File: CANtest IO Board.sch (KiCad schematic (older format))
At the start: 40 parts, among them J1 Inputs, J2 Conn_02x16_Counter_Clockwise, J3 Outputs, SW1 SW_SPDT_MSM, SW2 SW_SPST, SW3 SW_SPST, SW4 SW_Push, SW5 SW_Push

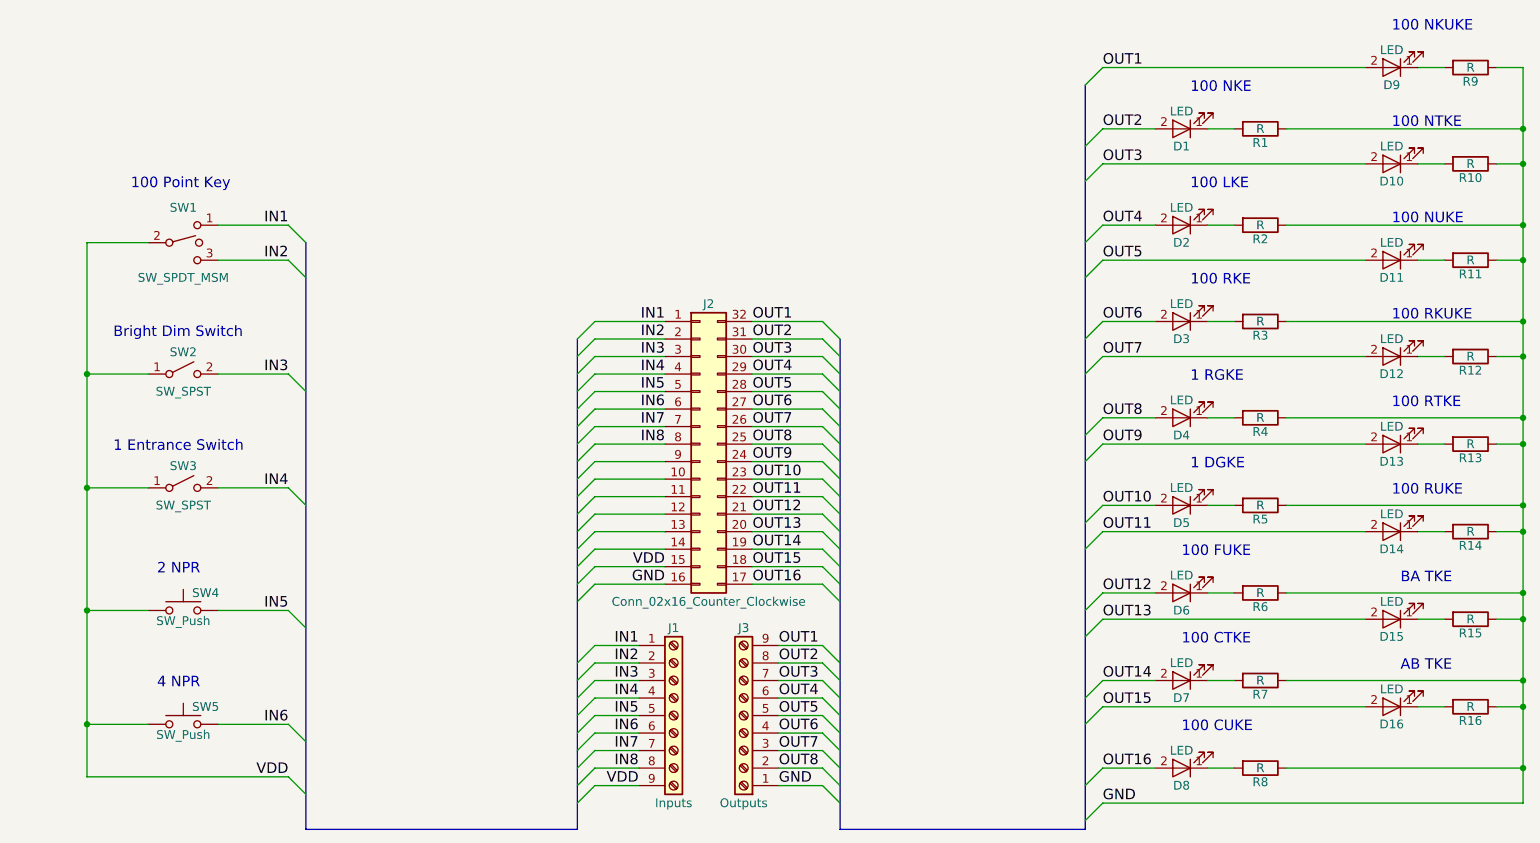
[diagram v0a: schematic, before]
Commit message: Progress
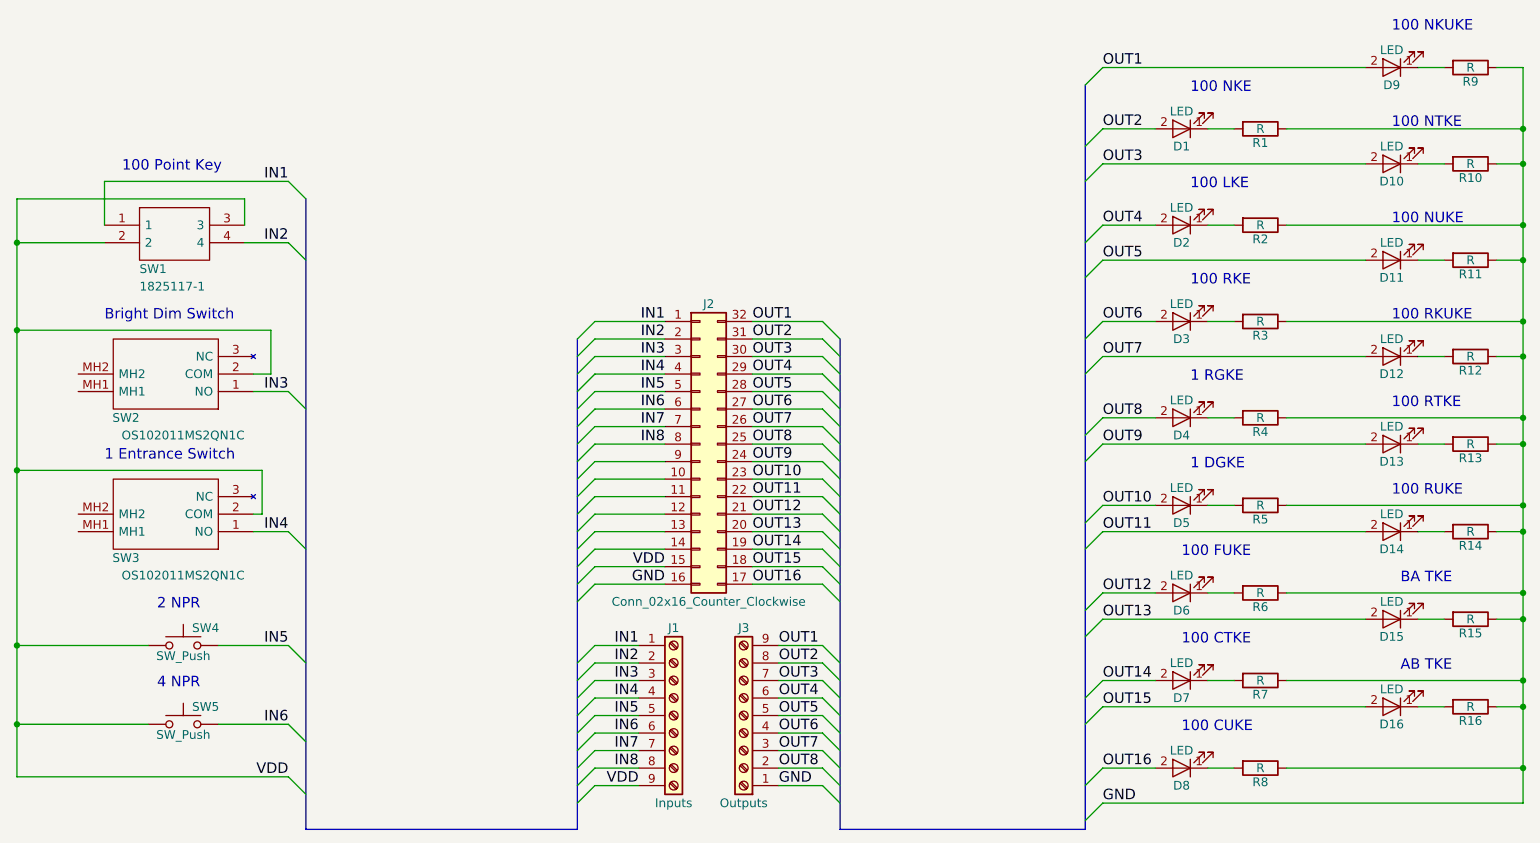
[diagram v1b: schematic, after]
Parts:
- removed SW1: SW_SPDT_MSM, symbol SW_SPDT_MSM
- removed SW2, SW3: SW_SPST, symbol SW_SPST
- added SW1: 1825117-1, SHDR4W87P0X320_1X4_1511X584X1100P, symbol 1825117-1
- added SW2, SW3: OS102011MS2QN1C, OS102011MS2QN1C, symbol OS102011MS2QN1C
- D1, D2, D3, D4, D5: footprint (none) -> LEDs:LED_D3.0mm_Horizontal_O1.27mm_Z6.0mm
- D10, D11, D12, D13, D14, D15, D16, D6, D7, D8, D9: footprint (none) -> LEDs:LED_Rectangular_W5.0mm_H2.0mm_Horizontal_O1.27mm_Z5.0mm
- J1, J3: footprint (none) -> TerminalBlocks_Phoenix:TerminalBlock_Phoenix_MPT-2.54mm_9pol
- J2: footprint (none) -> Pin_Headers:Pin_Header_Angled_2x16_Pitch2.54mm
- R1, R10, R11, R12, R13, R14, R15, R16, R2, R3, R4, R5, R6, R7, R8, R9: footprint (none) -> Resistors_SMD:R_0805_HandSoldering
- SW4, SW5: footprint (none) -> Buttons_Switches_SMD:SW_SPST_KMR2
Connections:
- net IN1: now also SW1.1
- net IN2: now also SW1.4
- net IN3: now also SW2.1 (NO)
- net IN4: now also SW3.1 (NO)
- net VDD: now also SW1.2, SW1.3, SW2.2 (COM), SW3.2 (COM)
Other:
- moved on the sheet: SW4
